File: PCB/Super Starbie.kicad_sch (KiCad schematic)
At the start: 15 parts, among them J1 Conn_01x04_Pin, J2 Conn_01x08_Pin, M1 Motor_DC, Q1 Q_NMOS_DGS, U3 DHT11

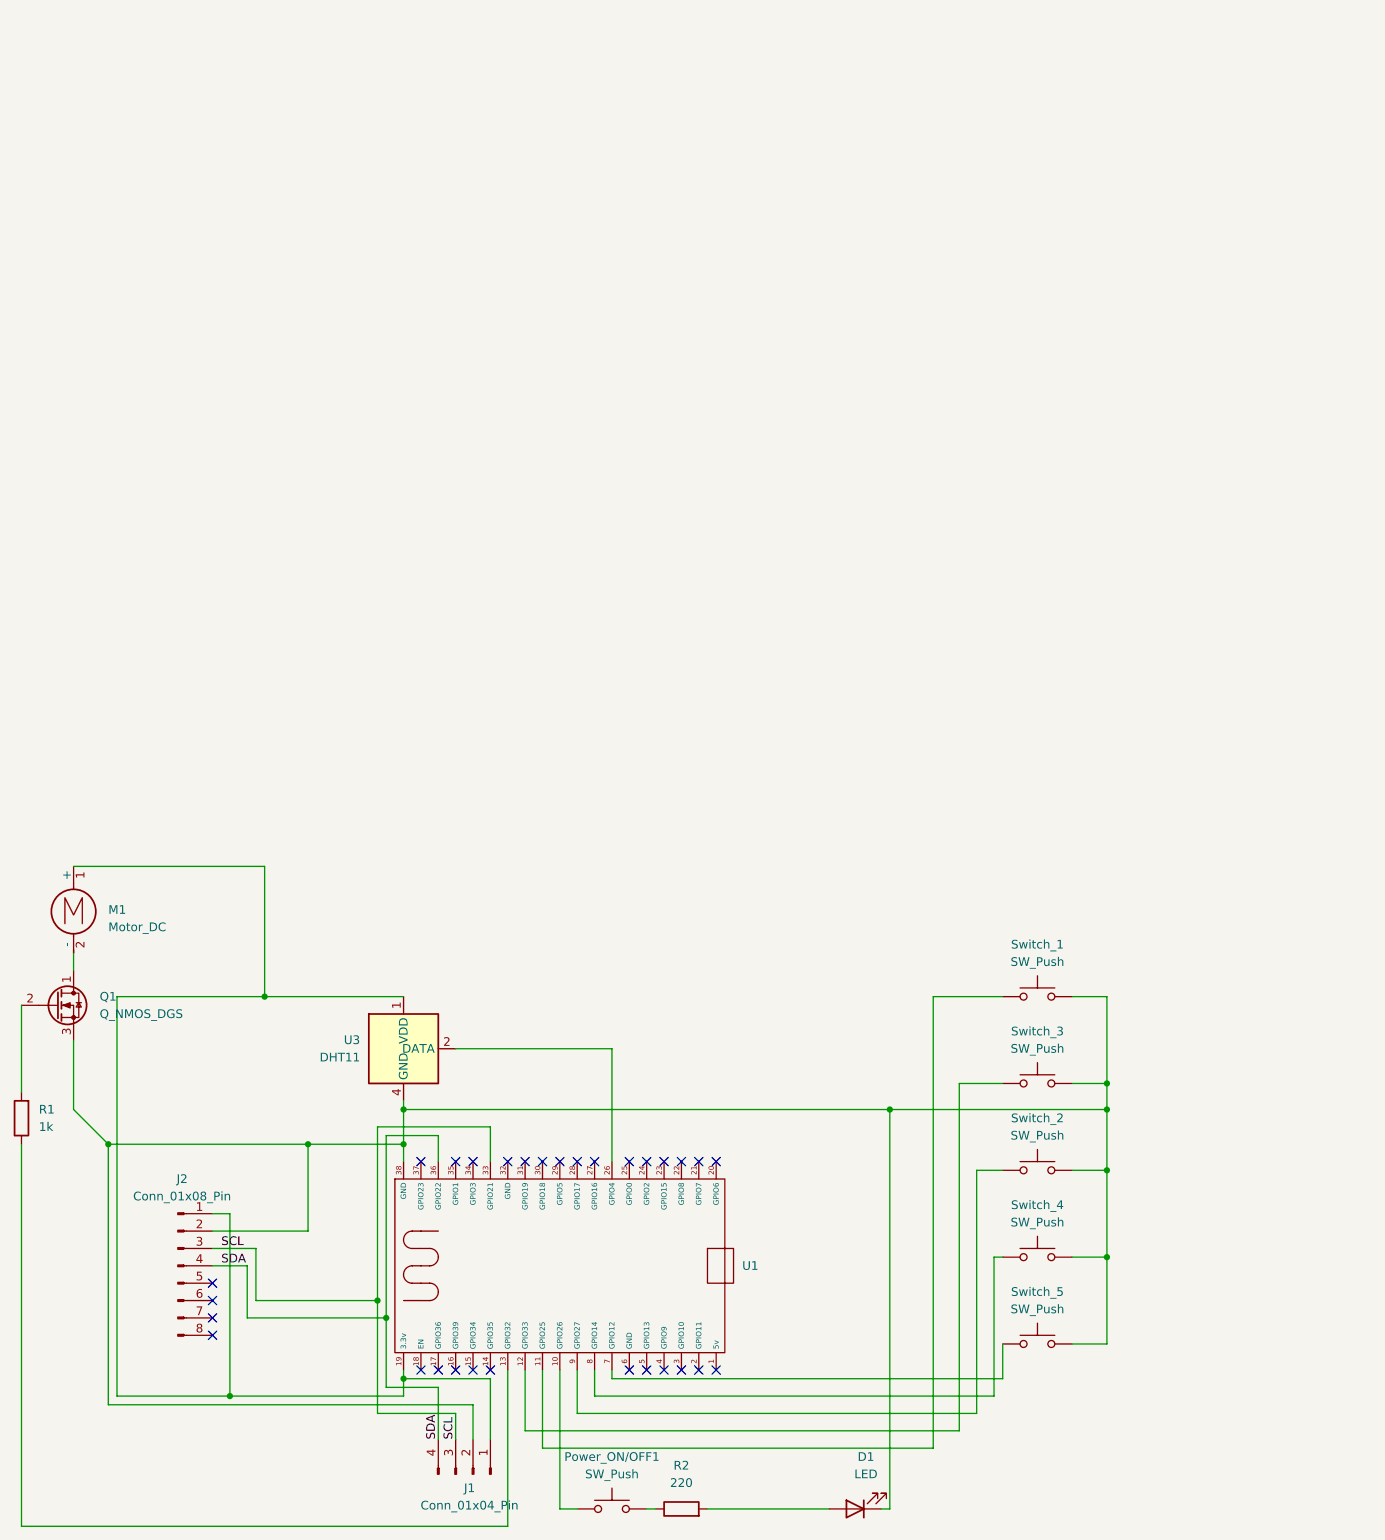
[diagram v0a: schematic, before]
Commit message: Add files via upload
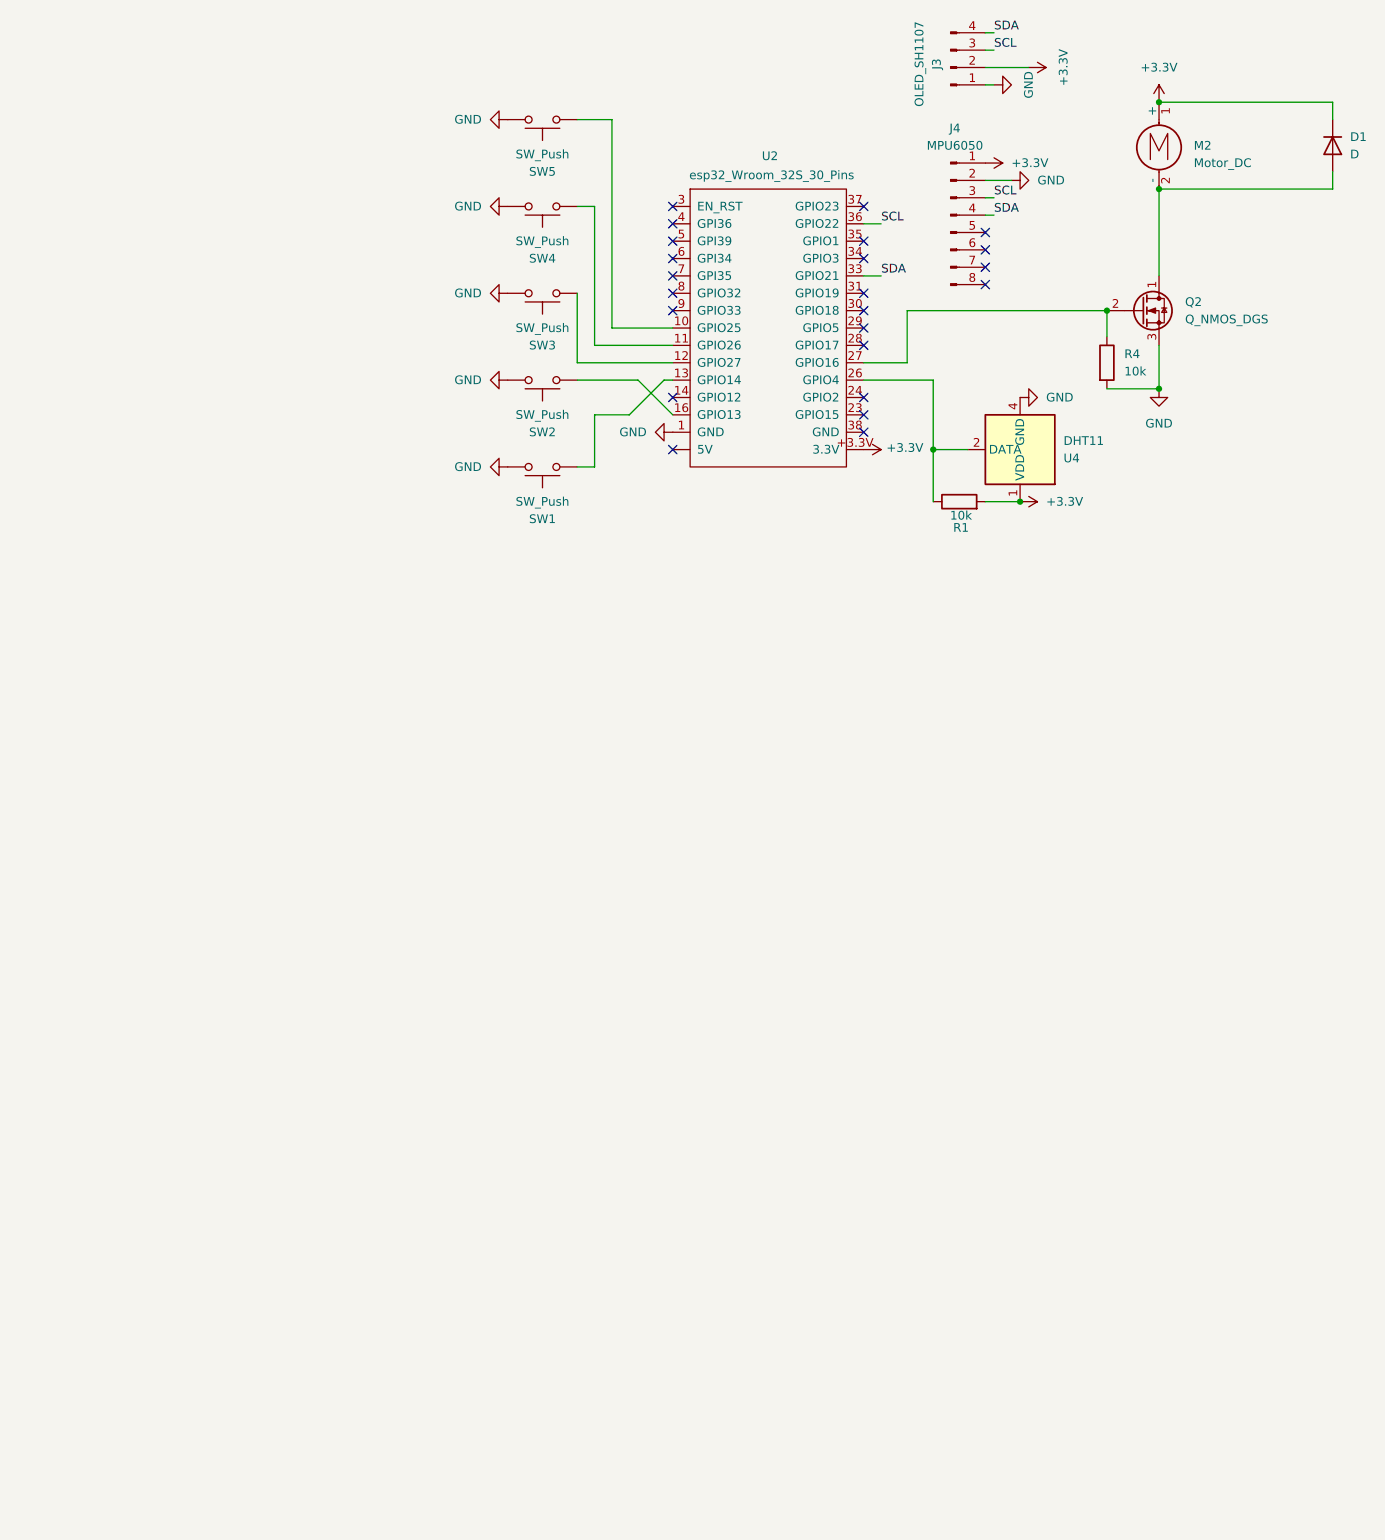
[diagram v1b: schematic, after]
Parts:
- removed D1: LED, LED_THT:LED_D5.0mm_Horizontal_O1.27mm_Z15.0mm, symbol Device:LED
- removed J1: Conn_01x04_Pin, Imported Parts:Display_128x64_096_I2C, symbol Connector:Conn_01x04_Pin
- removed J2: Conn_01x08_Pin, Connector_PinHeader_2.54mm:PinHeader_1x08_P2.54mm_Vertical, symbol Connector:Conn_01x08_Pin
- removed M1: Motor_DC, Connector_PinHeader_2.54mm:PinHeader_1x02_P2.54mm_Vertical, symbol Motor:Motor_DC
- removed Power_ON/OFF1, Switch_1, Switch_2, Switch_3, Switch_4, Switch_5: SW_Push, Button_Switch_THT:SW_PUSH_6mm, symbol Switch:SW_Push
- removed Q1: Q_NMOS_DGS, Package_TO_SOT_THT:TO-220-3_Vertical, symbol Transistor_FET:Q_NMOS_DGS
- removed R2: 220, Resistor_THT:R_Axial_DIN0204_L3.6mm_D1.6mm_P7.62mm_Horizontal, symbol Device:R
- removed U1: (no value), ESP32_38pin, symbol esp32_38pin:ESP32_38Pin
- removed U3: DHT11, Sensor:Aosong_DHT11_5.5x12.0_P2.54mm, symbol Sensor:DHT11
- added D1: D, Diode_THT:D_DO-35_SOD27_P7.62mm_Horizontal, symbol Device:D
- added J3: OLED_SH1107, Imported Parts:Display_128x64_096_I2C, symbol Connector:Conn_01x04_Pin
- added J4: MPU6050, Connector_PinHeader_2.54mm:PinHeader_1x08_P2.54mm_Vertical, symbol Connector:Conn_01x08_Pin
- added M2: Motor_DC, Connector_PinHeader_2.54mm:PinHeader_1x02_P2.54mm_Vertical, symbol Motor:Motor_DC
- added Q2: Q_NMOS_DGS, Package_TO_SOT_THT:TO-220-3_Vertical, symbol Transistor_FET:Q_NMOS_DGS
- added R4: 10k, Resistor_THT:R_Axial_DIN0204_L3.6mm_D1.6mm_P7.62mm_Horizontal, symbol Device:R
- added SW1, SW2, SW3, SW4, SW5: SW_Push, Button_Switch_Keyboard:SW_Cherry_MX_1.00u_PCB, symbol Switch:SW_Push
- added U2: esp32_Wroom_32S_30_Pins, Calibration_Scale:THE NEW FOOTPRINTER, symbol New_Library_0:esp32_38_pins-custom_library
- added U4: DHT11, Sensor:Aosong_DHT11_5.5x12.0_P2.54mm, symbol Sensor:DHT11
- R1: value 1k -> 10k
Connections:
- net SCL: now also J3.3 (Pin_3), J4.3 (Pin_3), U2.36 (GPIO22)
- net SDA: now also J3.4 (Pin_4), J4.4 (Pin_4), U2.33 (GPIO21)
- net at R1.1: now also U2.26 (GPIO4), U4.2 (DATA)
- net +3.3V: now reaches R1.2
- net +3.3V: now also D1.1 (K), J3.2 (Pin_2), J4.1 (Pin_1), M2.1 (+), U2.+3.3V (3.3V), U4.1 (VDD)
- new net: D1.2 (A), M2.2 (-), Q2.1 (D)
- new net: SW1.1, U2.13 (GPIO14)
- new net: SW3.1, U2.12 (GPIO27)
- new net: SW4.1, U2.11 (GPIO26)
- new net: SW2.1, U2.16 (GPIO13)
- new net: SW5.1, U2.10 (GPIO25)
- new net: Q2.2 (G), R4.1, U2.27 (GPIO16)
- new net GND: J3.1 (Pin_1), J4.2 (Pin_2), Q2.3 (S), R4.2, SW1.2, SW2.2, SW3.2, SW4.2, SW5.2, U2.1 (GND), U4.4 (GND)
- no-connect marks 30 -> 23
